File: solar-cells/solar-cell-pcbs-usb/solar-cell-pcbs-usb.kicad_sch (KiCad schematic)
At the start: 18 parts, among them J1 Solar Cell, J2 Burn Wire

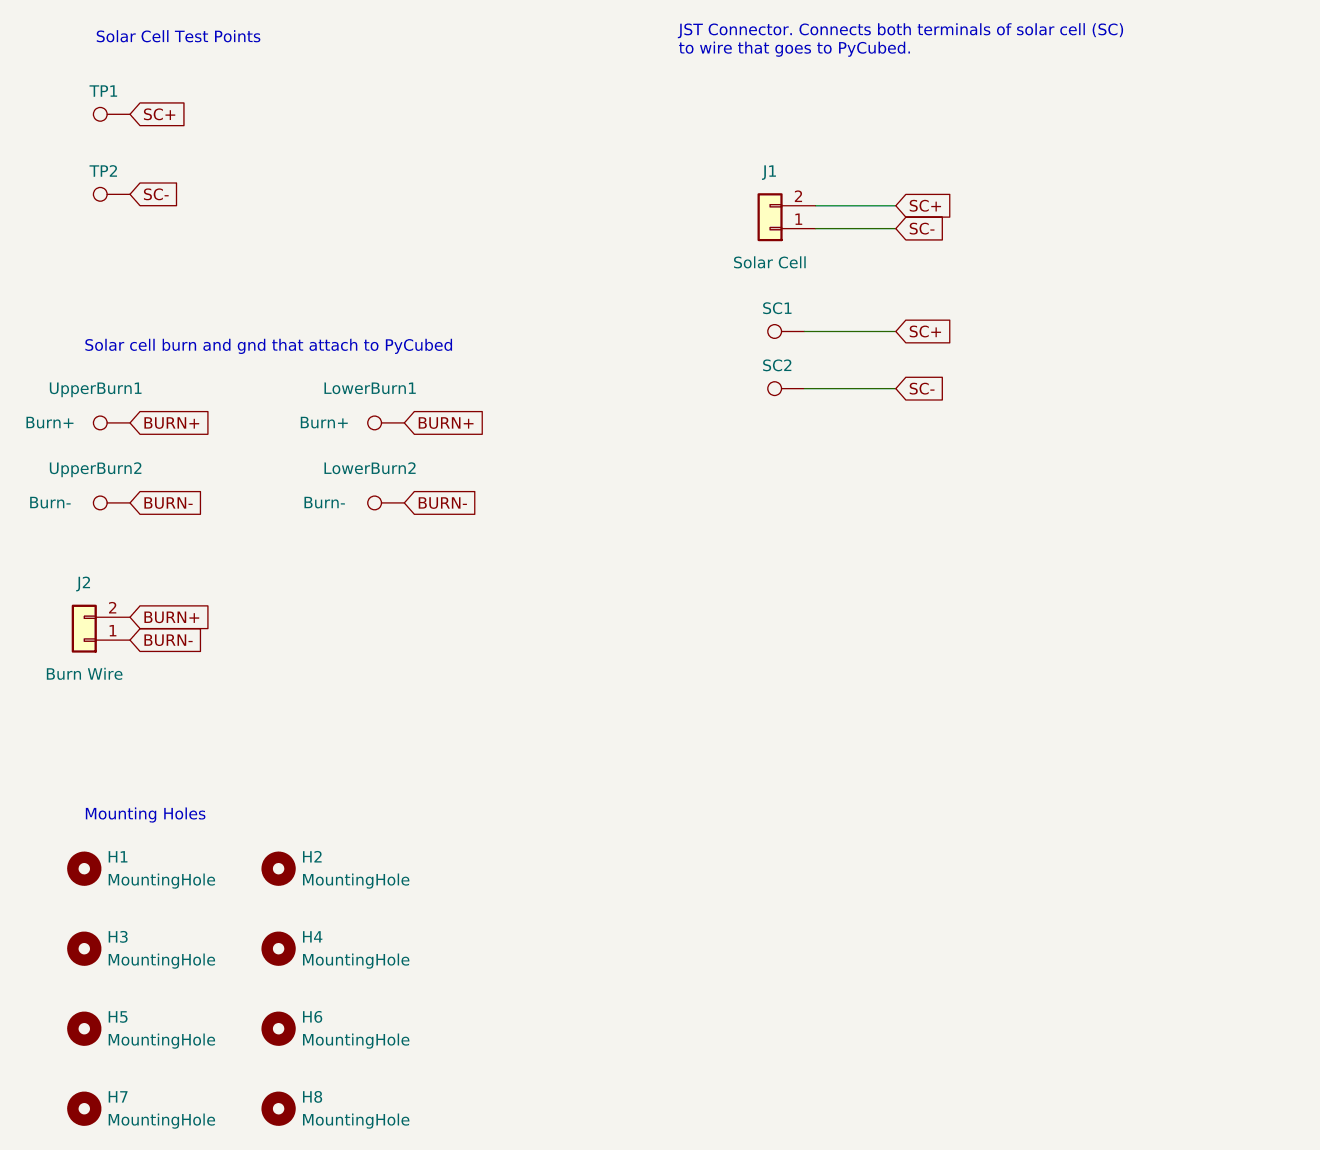
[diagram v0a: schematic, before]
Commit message: modifications to solar cell folder
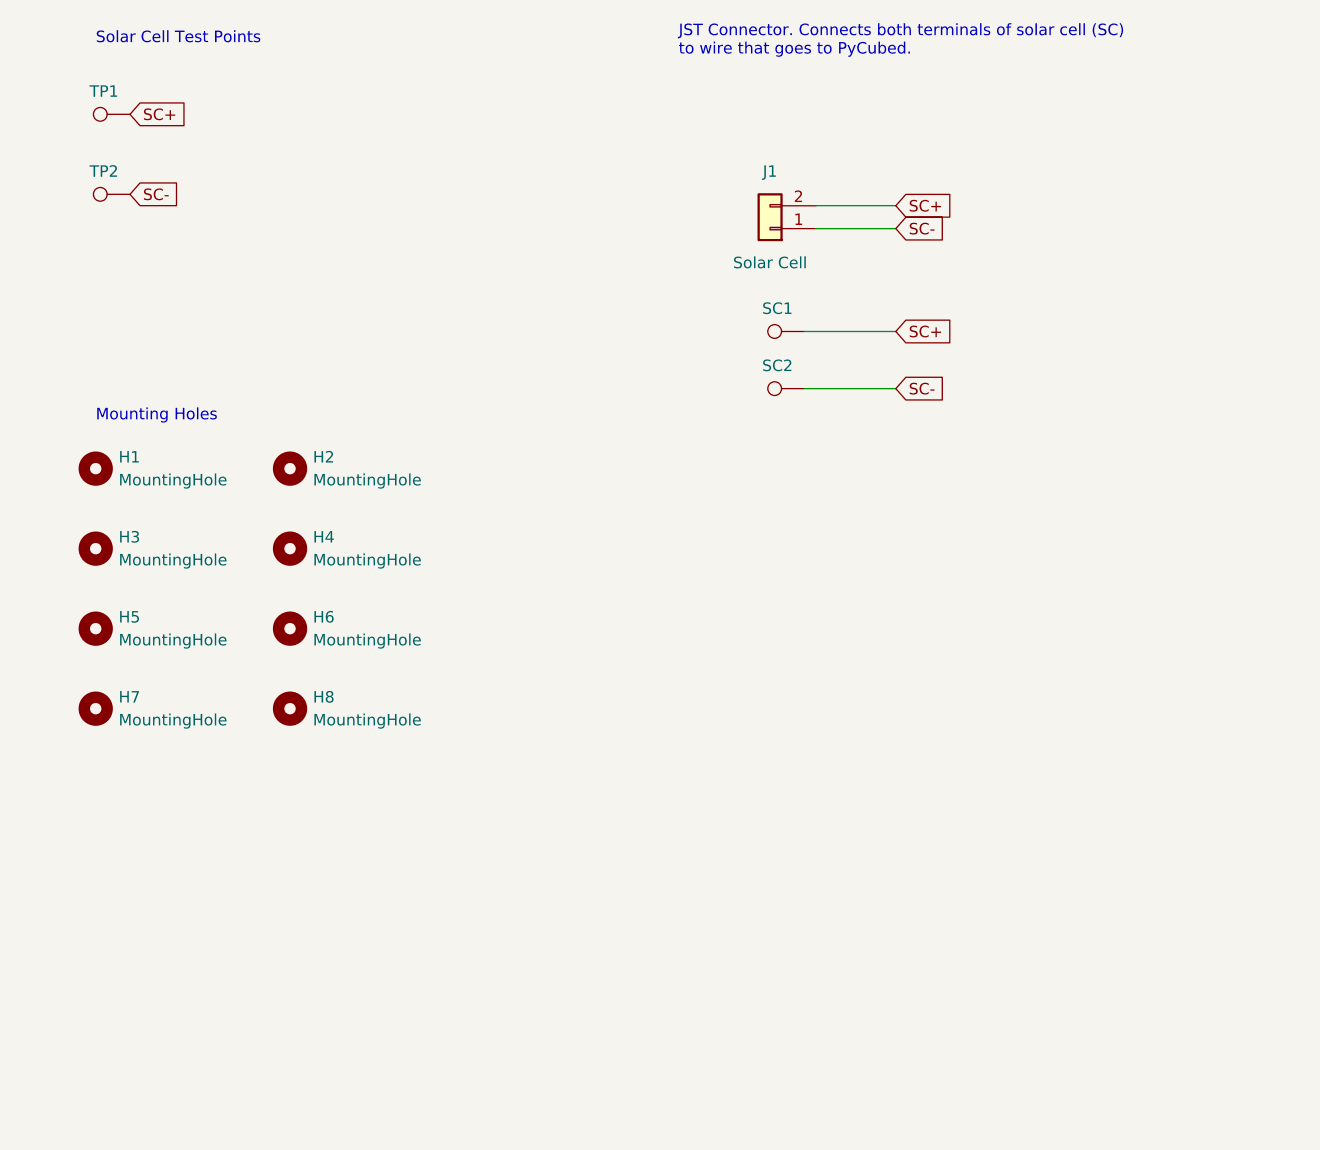
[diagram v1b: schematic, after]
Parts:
- removed J2: Burn Wire, Molex_PicoLock_2p_2mm_2053380002:2053380002, symbol Connector_Generic:Conn_01x02
- removed LowerBurn1, UpperBurn1: Burn+, TestPoint:TestPoint_Pad_2.0x2.0mm, symbol Connector:TestPoint
- removed LowerBurn2, UpperBurn2: Burn-, TestPoint:TestPoint_Pad_2.0x2.0mm, symbol Connector:TestPoint
- SC1, SC2: footprint TestPoint:TestPoint_Pad_D3.0mm -> TestPoint:TestPoint_THTPad_D3.0mm_Drill1.5mm
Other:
- note removed: "Solar cell burn and gnd that attach to PyCubed"
- moved on the sheet: H1, H2, H3, H4, H5, H6, H7, H8
